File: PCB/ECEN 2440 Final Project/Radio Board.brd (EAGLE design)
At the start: 39 x 54.6 mm, 12 parts

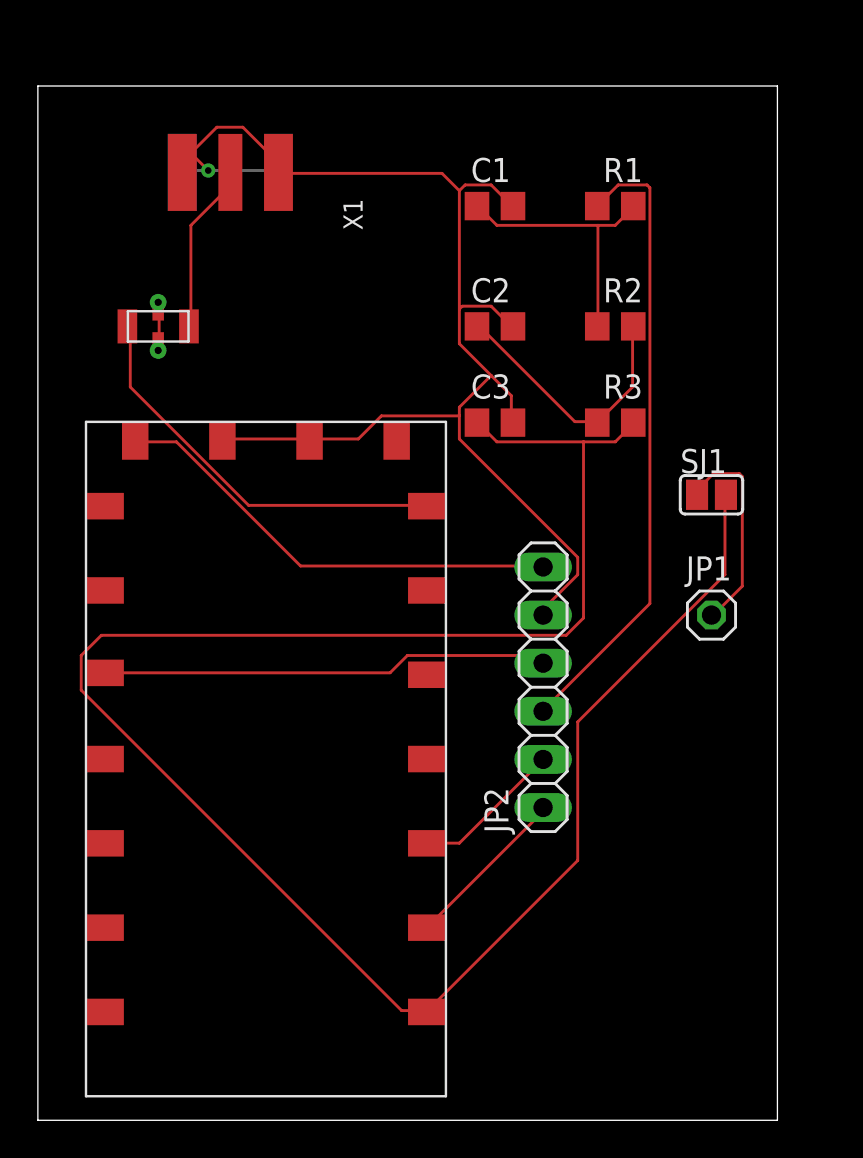
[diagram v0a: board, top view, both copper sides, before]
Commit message: minor changes to board
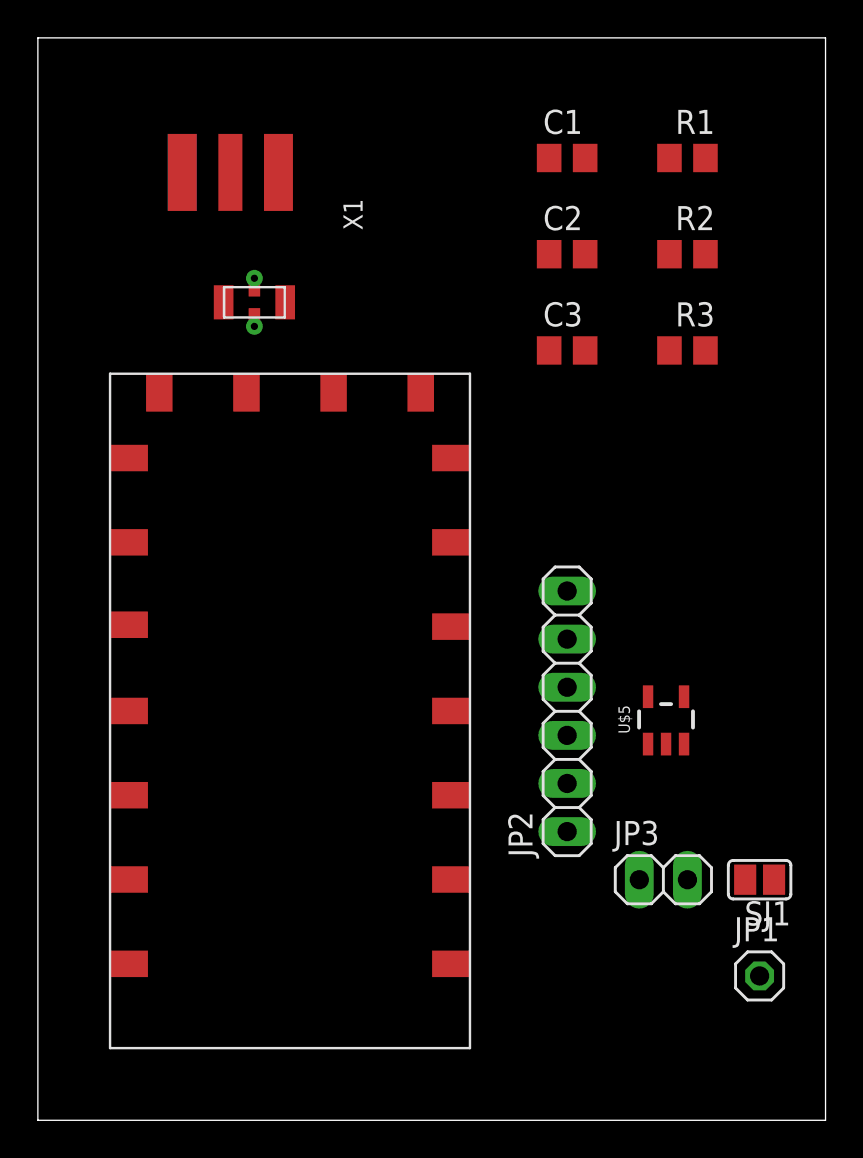
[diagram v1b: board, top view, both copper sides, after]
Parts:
- added JP3: (no value), pinhead:1X02
- added U$5: LDO-S-816, Custom Library:LDO-S-816
- moved SJ1 20.5 mm to (38.1, 12.7), turned to 180 degrees
- moved JP1 19.2 mm to (38.1, 7.62)
- moved C2 5.39 mm to (27.9, 45.7)
- moved C3 5.39 mm to (27.9, 40.6)
- moved R2 5.39 mm to (34.3, 45.7)
- moved R3 5.39 mm to (34.3, 40.6)
- moved U$6 5.24 mm to (11.4, 43.2), turned to 180 degrees
- moved C1 4.58 mm to (27.9, 50.8)
- moved R1 4.58 mm to (34.3, 50.8)
- moved U$4 2.84 mm to (3.81, 3.81)
- moved JP2 1.80 mm to (27.9, 21.6)
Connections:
- new net VCC: JP3.2, U$5.VIN
- net GND: now also JP3.1, U$5.VSS
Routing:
- net N$5: track 106.4 -> 0.00 mm
- net GND: track 75.3 -> 0.00 mm, vias 1 -> 0
- net AUDIO_PWM: track 33.3 -> 0.00 mm
- net +3V3: track 24.3 -> 0.00 mm
- net AUDIO_PTT: track 23.7 -> 0.00 mm
- net N$1: track 21.6 -> 0.00 mm
- net N$2: track 14.5 -> 0.00 mm
- net N$4: track 14.3 -> 0.00 mm
- net N$3: track 11.1 -> 0.00 mm
- net N$6: track 9.11 -> 0.00 mm
- net TX_RADIO: track 8.88 -> 0.00 mm
- net RX_RADIO: track 7.96 -> 0.00 mm
- net GND1: track 3.29 -> 0.00 mm
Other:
- board size 39 x 54.6 mm -> 41.6 x 57.1 mm
